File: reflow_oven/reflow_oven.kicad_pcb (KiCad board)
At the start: 2 copper layers, 49 x 58.2 mm, 30 parts, among them J1 UART, J2 POWER, J3 LED, J4 K-TYPE, J5 BUTTON1, J6 BUTTON2, J7 RELAY, J8 I2C, Q1 2n2222, U1 ATmega328-PU, U2 MAX6675, Y1 16MHz

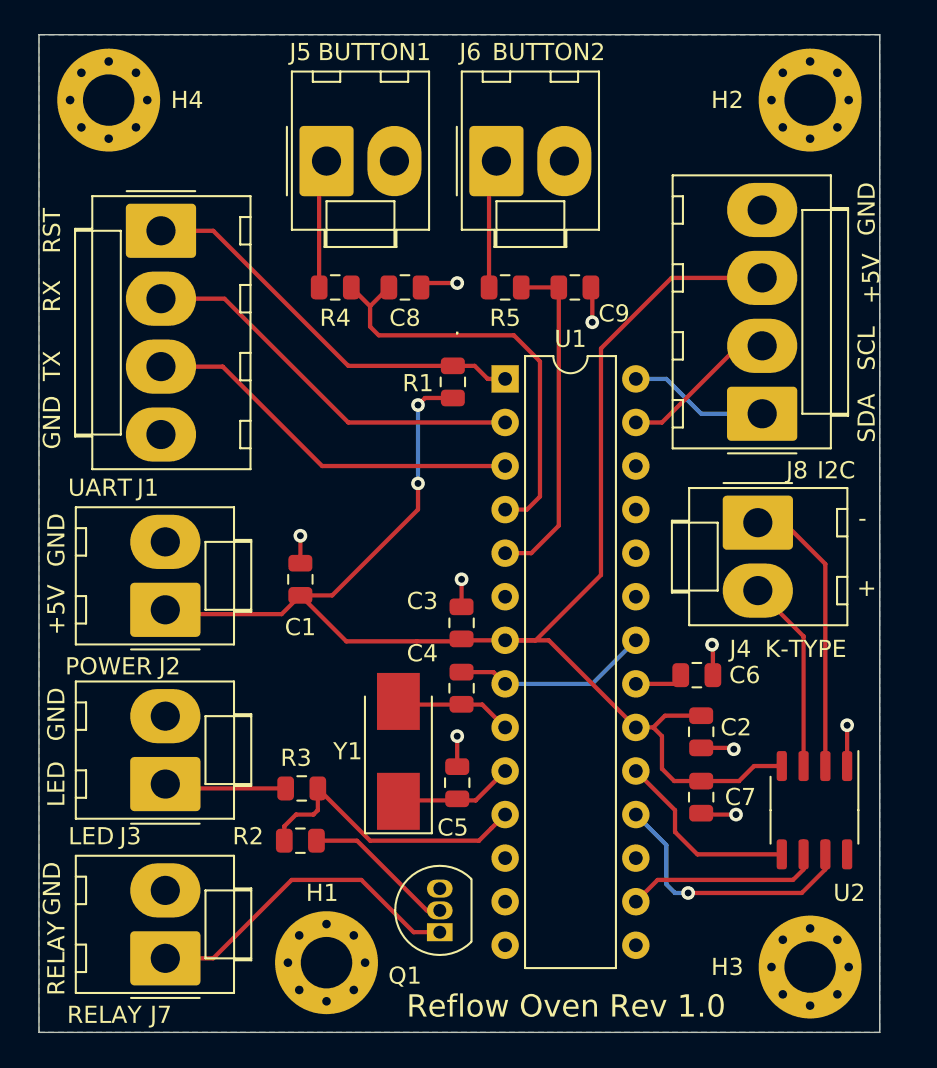
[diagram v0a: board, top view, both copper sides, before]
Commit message: Updated Design
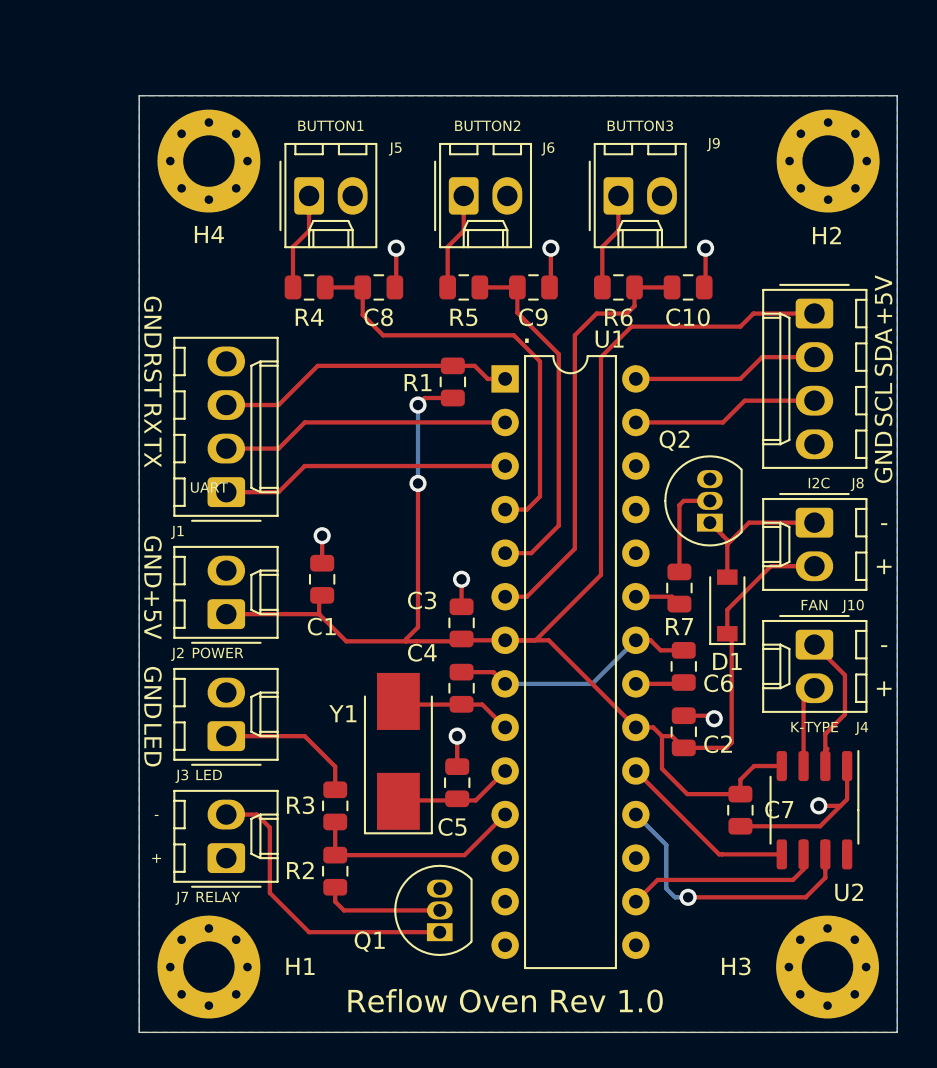
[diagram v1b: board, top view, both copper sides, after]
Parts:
- added C10: 100n, Capacitor_SMD:C_0805_2012Metric, F.Cu at (60.7, 62.2)
- added D1: MBR0540T1G, Diode_SMD:D_SOD-123, F.Cu at (63.0, 80.8)
- added J10: FAN, Connector_Molex:Molex_KK-254_AE-6410-02A_1x02_P2.54mm_Vertical, F.Cu at (68.1, 75.9)
- added J9: BUTTON3, Connector_Molex:Molex_KK-254_AE-6410-02A_1x02_P2.54mm_Vertical, F.Cu at (56.6, 56.9)
- added Q2: 2n2222, Package_TO_SOT_THT:TO-92_Inline, F.Cu at (62.0, 75.9)
- added R6: 1k, Resistor_SMD:R_0805_2012Metric, F.Cu at (56.6, 62.2)
- added R7: 1k, Resistor_SMD:R_0805_2012Metric, F.Cu at (60.2, 79.8)
- J1, J8: footprint Connector_Molex:Molex_KK-396_A-41791-0004_1x04_P3.96mm_Vertical -> Connector_Molex:Molex_KK-254_AE-6410-04A_1x04_P2.54mm_Vertical
- J2, J3, J4, J5, J6, J7: footprint Connector_Molex:Molex_KK-396_A-41791-0002_1x02_P3.96mm_Vertical -> Connector_Molex:Molex_KK-254_AE-6410-02A_1x02_P2.54mm_Vertical
- moved J1 15.7 mm to (33.8, 74.2), turned to 90 degrees
- moved J4 7.84 mm to (68.1, 83.1)
- moved H1 6.86 mm to (32.8, 101.9)
- moved H4 6.84 mm to (32.8, 54.9)
- moved J7 6.84 mm to (33.8, 95.5)
- moved J8 6.59 mm to (68.1, 63.8), turned to 270 degrees
- moved J3 4.52 mm to (33.8, 88.4)
- moved H2 3.71 mm to (68.9, 54.9)
- moved J2 3.57 mm to (33.8, 81.3)
- moved J6 2.79 mm to (47.6, 56.9)
- moved R2 2.70 mm to (40.1, 96.3), turned to 90 degrees
- moved C9 2.41 mm to (51.7, 62.2)
- moved R5 2.41 mm to (47.6, 62.2)
- moved C7 2.41 mm to (63.8, 92.7)
- moved J5 2.27 mm to (38.6, 56.9)
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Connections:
- C1 pad 1: +5V -> FAN_CONN+
- C2 pad 1: +5V -> FAN_CONN+
- C3 pad 1: +5V -> FAN_CONN+
- C7 pad 1: +5V -> FAN_CONN+
- J1 pad 1: RST -> UART_TX
- J1 pad 3: UART_TX -> RST
- J2 pad 1: +5V -> FAN_CONN+
- J7 pad 1: RELAY_CONN -> FAN_CONN+
- J7 pad 2: GND -> RELAY_CONN
- J8 pad 1: SDA -> FAN_CONN+
- J8 pad 2: SCL -> SDA
- J8 pad 3: +5V -> SCL
- R1 pad 1: +5V -> FAN_CONN+
- U1 pad 20: +5V -> FAN_CONN+
- U1 pad 23: Net-(U1-Pad23) -> FAN
- U1 pad 6: Net-(U1-Pad6) -> BUTTON3
- U1 pad 7: +5V -> FAN_CONN+
- U2 pad 4: +5V -> FAN_CONN+
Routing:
- net FAN_CONN+: track 0.00 -> 107.7 mm, vias 0 -> 2
- net +5V: track 94.7 -> 0.00 mm, vias 2 -> 0
- net BUTTON3: track 0.00 -> 25.1 mm
- net FAN_CONN-: track 0.00 -> 9.20 mm
- net GND: track 28.3 -> 37.5 mm, vias 9 -> 8
- net K-: track 16.7 -> 9.34 mm
- net K+: track 11.3 -> 4.98 mm
- net UART_RX: track 23.1 -> 16.9 mm
- net RST: track 23.6 -> 17.5 mm
- net Net-(Q2-Pad2): track 0.00 -> 5.77 mm
- net BUTTON3_CONN: track 0.00 -> 5.72 mm
- net UART_TX: track 22.5 -> 16.9 mm
- net RELAY: track 17.3 -> 12.8 mm
- net FAN: track 0.00 -> 2.72 mm
- net BUTTON2_CONN: track 7.80 -> 5.72 mm
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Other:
- board size 49 x 58.2 mm -> 44.2 x 54.6 mm
- board text added: "BUTTON3"
- board text added: "FAN"
